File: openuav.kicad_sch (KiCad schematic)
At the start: 32 parts, among them U1 STM32G431CBUx, U2 AT7456E, U3 LSM6DSR, U4 LPS22HH, U5 L78L33_SOT89, U6 W25N01GVZEIG, U7 L78L05_SOT89, U8 L78L09_SOT89

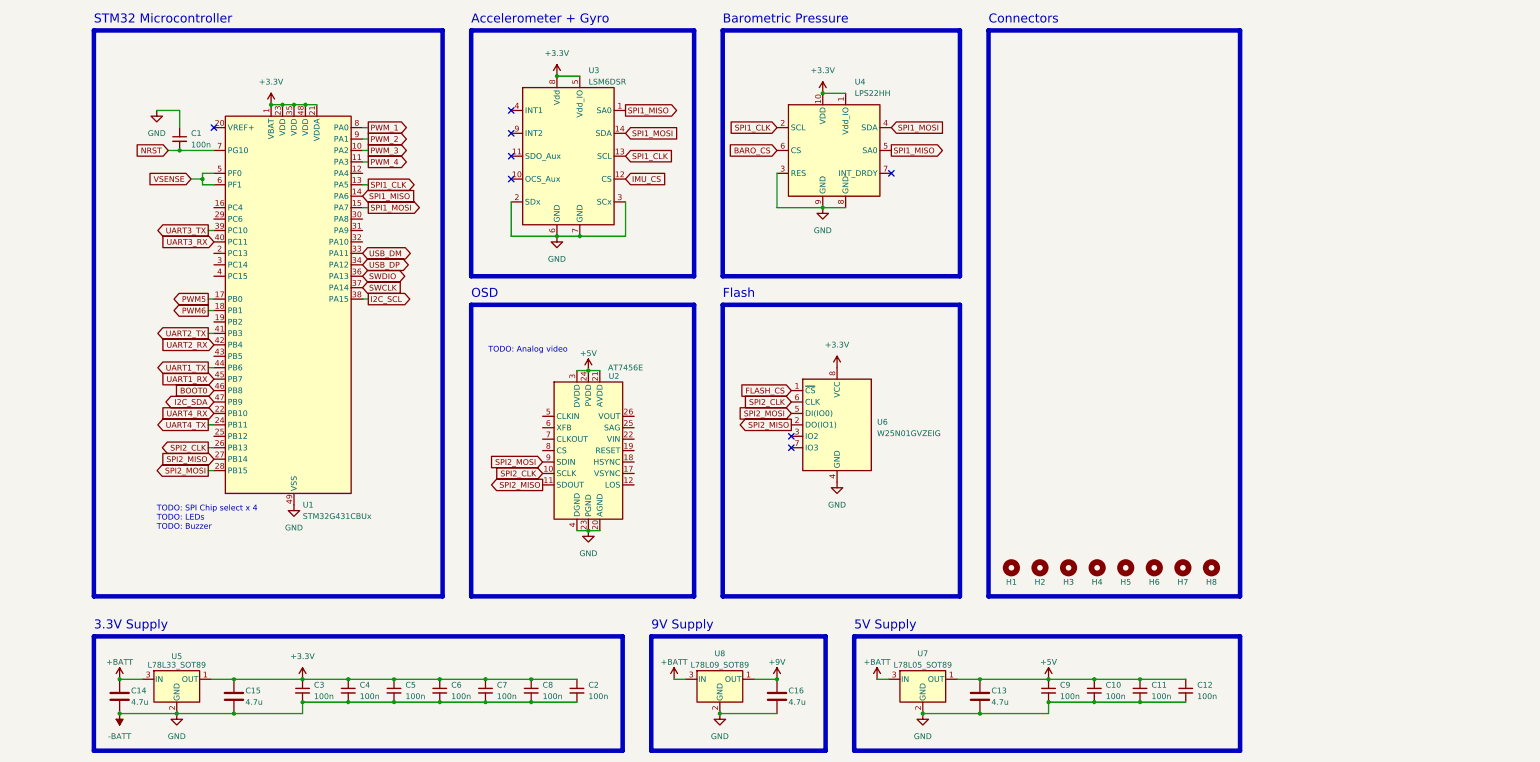
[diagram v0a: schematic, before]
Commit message: Continued work in progress on initial design
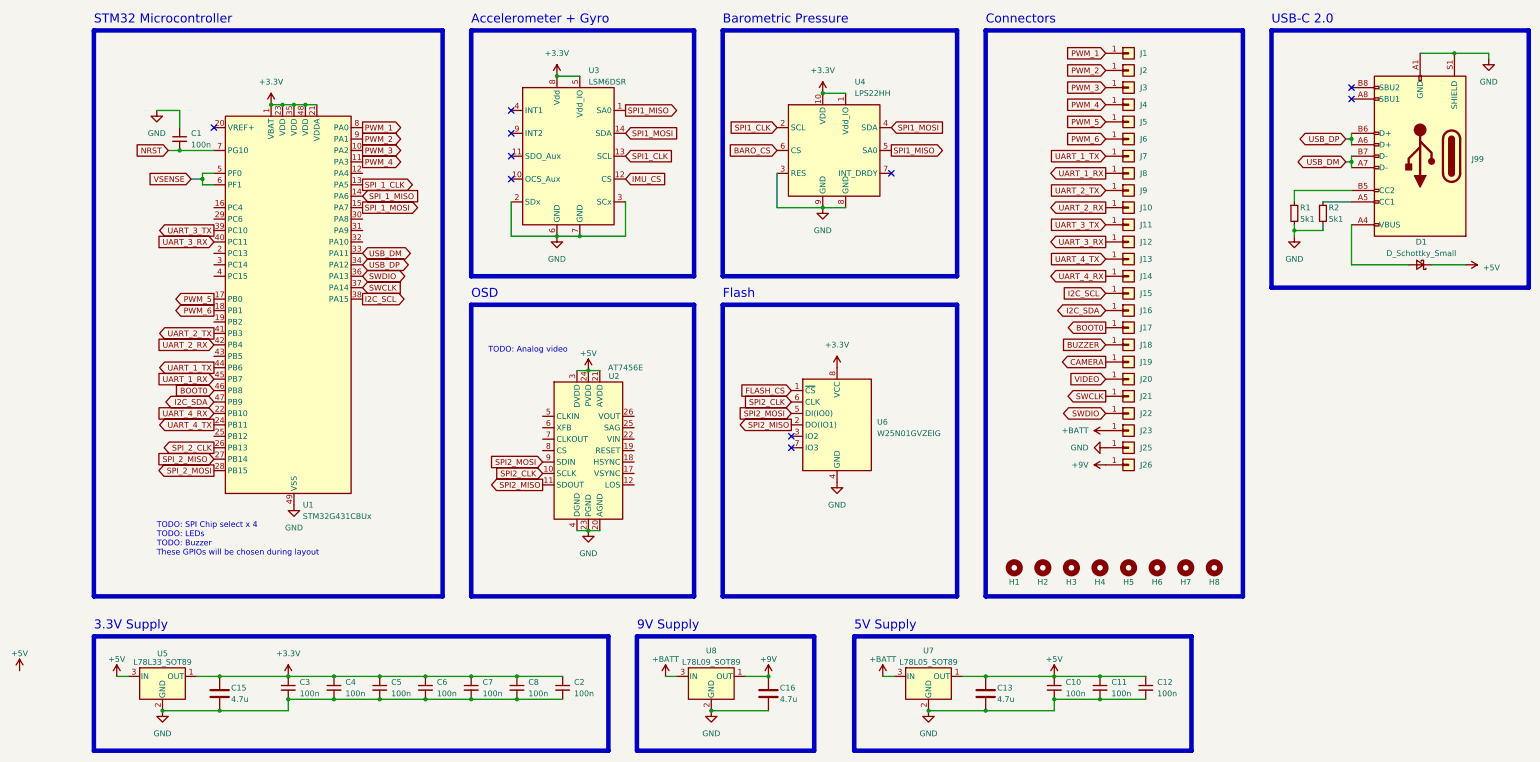
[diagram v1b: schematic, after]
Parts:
- removed C14: 4.7u, Capacitor_SMD:C_0603_1608Metric, symbol Device:C
- removed C9: 100n, Capacitor_SMD:C_0402_1005Metric, symbol Device:C_Small
- added D1: D_Schottky_Small, symbol Device:D_Schottky_Small
- added J1, J10, J11, J12, J13, J14, J15, J16, J17, J18, J19, J2, J20, J21, J22, J23, J25, J26, J3, J4, J5, J6, J7, J8, J9: Conn_01x01, TestPoint:TestPoint_Pad_2.0x2.0mm, symbol Connector_Generic:Conn_01x01
- added J99: USB_C_Receptacle_USB2.0, Connector_USB:USB_C_Receptacle_XKB_U262-16XN-4BVC11, symbol Connector:USB_C_Receptacle_USB2.0
- added R1, R2: 5k1, symbol Device:R_Small
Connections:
- net +5V: now also U5.3 (IN), D1.1 (K)
- net +9V: now also J26.1 (Pin_1)
- net +BATT: now also J23.1 (Pin_1); no longer U5.3 (IN)
- net BOOT0: now also J17.1 (Pin_1)
- net I2C_SCL: now also J15.1 (Pin_1)
- net I2C_SDA: now also J16.1 (Pin_1)
- net PWM_1: now also J1.1 (Pin_1)
- net PWM_2: now also J2.1 (Pin_1)
- net PWM_3: now also J3.1 (Pin_1)
- net PWM_4: now also J4.1 (Pin_1)
- net SPI1_CLK: no longer U1.13 (PA5)
- net SPI1_MISO: no longer U1.14 (PA6)
- net SPI1_MOSI: no longer U1.15 (PA7)
- net SPI2_CLK: no longer U1.26 (PB13)
- net SPI2_MISO: no longer U1.27 (PB14)
- net SPI2_MOSI: no longer U1.28 (PB15)
- net SWCLK: now also J21.1 (Pin_1)
- net SWDIO: now also J22.1 (Pin_1)
- net USB_DM: now also J99.A7 (D-), J99.B7 (D-)
- net USB_DP: now also J99.A6 (D+), J99.B6 (D+)
- net -BATT renamed GND
- net GND: now also J25.1 (Pin_1), J99.A1 (GND), J99.A12 (GND), J99.B1 (GND), J99.B12 (GND), J99.S1 (SHIELD), R1.2, R2.2
- net PWM5 renamed PWM_5
- net PWM_5: now also J5.1 (Pin_1)
- net PWM6 renamed PWM_6
- net PWM_6: now also J6.1 (Pin_1)
- net UART1_RX renamed UART_1_RX
- net UART_1_RX: now also J8.1 (Pin_1)
- net UART1_TX renamed UART_1_TX
- net UART_1_TX: now also J7.1 (Pin_1)
- net UART2_RX renamed UART_2_RX
- net UART_2_RX: now also J10.1 (Pin_1)
- net UART2_TX renamed UART_2_TX
- net UART_2_TX: now also J9.1 (Pin_1)
- net UART3_RX renamed UART_3_RX
- net UART_3_RX: now also J12.1 (Pin_1)
- net UART3_TX renamed UART_3_TX
- net UART_3_TX: now also J11.1 (Pin_1)
- net UART4_RX renamed UART_4_RX
- net UART_4_RX: now also J14.1 (Pin_1)
- net UART4_TX renamed UART_4_TX
- net UART_4_TX: now also J13.1 (Pin_1)
- new net: J99.B5 (CC2), R1.1
- new net: J99.A5 (CC1), R2.1
- new net: D1.2 (A), J99.A4 (VBUS), J99.A9 (VBUS), J99.B4 (VBUS), J99.B9 (VBUS)
- new net BUZZER: J18.1 (Pin_1)
- new net CAMERA: J19.1 (Pin_1)
- new net SPI_1_CLK: U1.13 (PA5)
- new net SPI_1_MISO: U1.14 (PA6)
- new net SPI_1_MOSI: U1.15 (PA7)
- new net SPI_2_CLK: U1.26 (PB13)
- new net SPI_2_MISO: U1.27 (PB14)
- new net SPI_2_MOSI: U1.28 (PB15)
- new net VIDEO: J20.1 (Pin_1)
- no-connect marks 8 -> 10
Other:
- note added: "TODO: SPI Chip select x 4 TODO: LEDs TODO: Buzzer These GPIOs will be chosen during layout"
- note added: "USB-C 2.0"
- note removed: "TODO: SPI Chip select x 4 TODO: LEDs TODO: Buzzer"
- moved on the sheet: C10, C11, C12, C13, C15, C16, C2, C3, C4, C5, C6, C7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
